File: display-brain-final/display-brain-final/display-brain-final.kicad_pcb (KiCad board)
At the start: 2 copper layers, 53 x 67.1 mm, 15 parts, among them J2 Conn_01x05_Socket, J3 Conn_01x19_Socket, J4 Conn_01x19_Socket, J5 Conn_01x04_Socket, J6 Conn_01x07_Socket, J7 Conn_01x02_Socket, P1 USB_C_Plug_USB2.0, U3 AMS1117CD-3.3

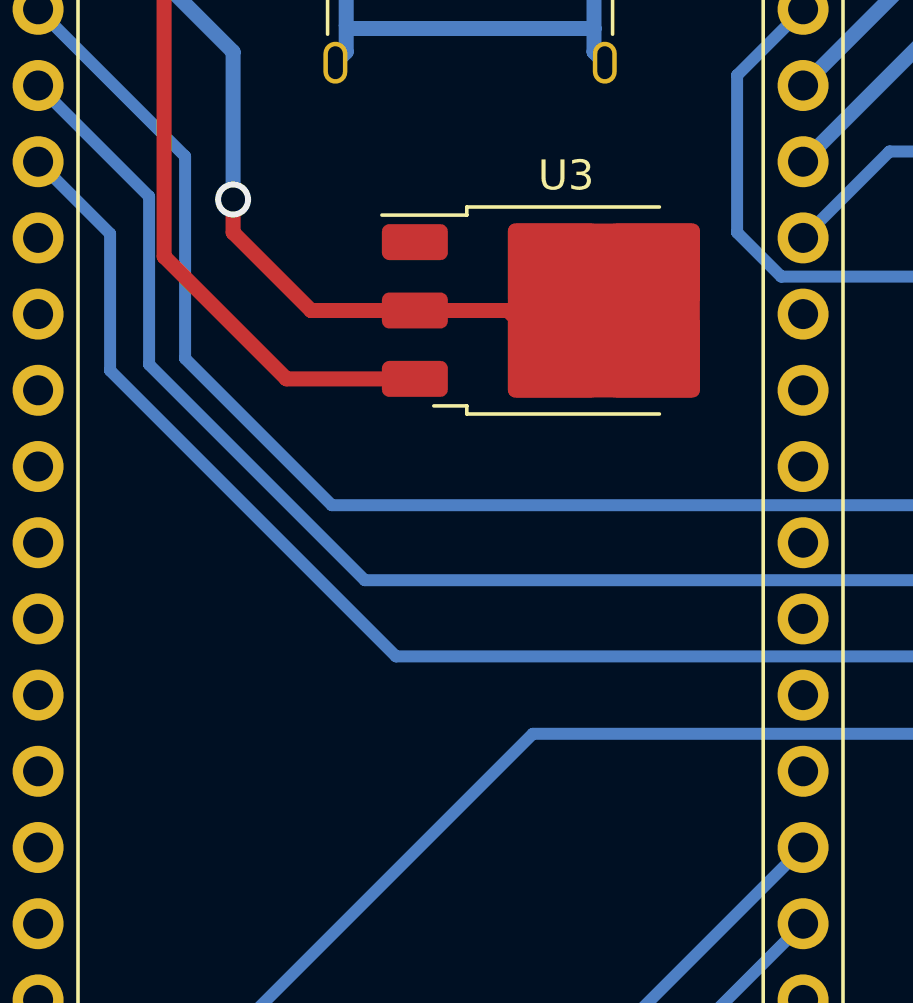
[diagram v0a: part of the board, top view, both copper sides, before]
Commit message: display brain platine fertig
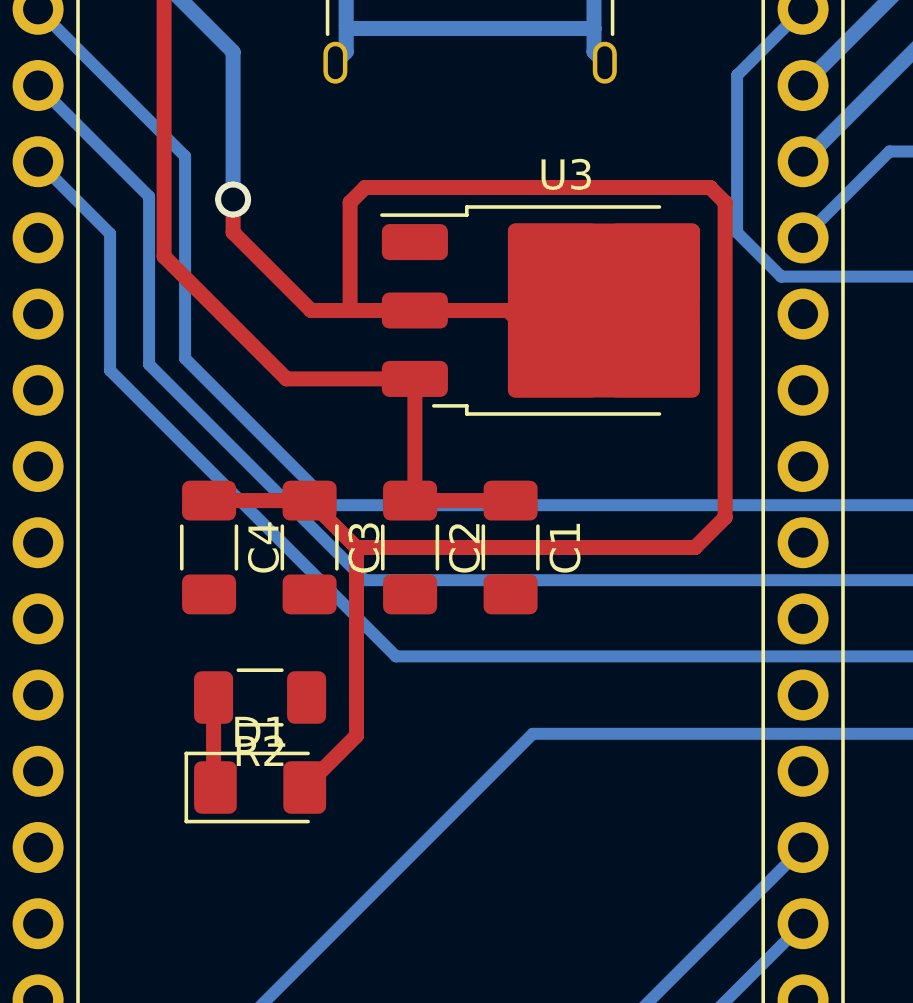
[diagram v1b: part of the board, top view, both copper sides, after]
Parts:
- added C1: 10u, Capacitor_SMD:C_1206_3216Metric_Pad1.33x1.80mm_HandSolder, F.Cu at (148.8, 83.5)
- added C2: 1u, Capacitor_SMD:C_1206_3216Metric_Pad1.33x1.80mm_HandSolder, F.Cu at (145.5, 83.5)
- added C3: 1u, Capacitor_SMD:C_1206_3216Metric_Pad1.33x1.80mm_HandSolder, F.Cu at (142.2, 83.5)
- added C4: 10u, Capacitor_SMD:C_1206_3216Metric_Pad1.33x1.80mm_HandSolder, F.Cu at (138.8, 83.5)
- added D1: LED, Diode_SMD:D_1206_3216Metric_Pad1.42x1.75mm_HandSolder, F.Cu at (140.5, 91.5)
- added R2: 330, Resistor_SMD:R_1206_3216Metric_Pad1.30x1.75mm_HandSolder, F.Cu at (140.5, 88.5)
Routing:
- net /3V3: track 27.6 -> 81.6 mm
- net Net-(U3-VI): track 45.6 -> 53.1 mm
- net Net-(D1-K): track 0.00 -> 3.03 mm
